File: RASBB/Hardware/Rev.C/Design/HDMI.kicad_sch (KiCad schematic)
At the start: 5 parts, among them IC11 TPD12S016PWR, J3 HDMI-001A

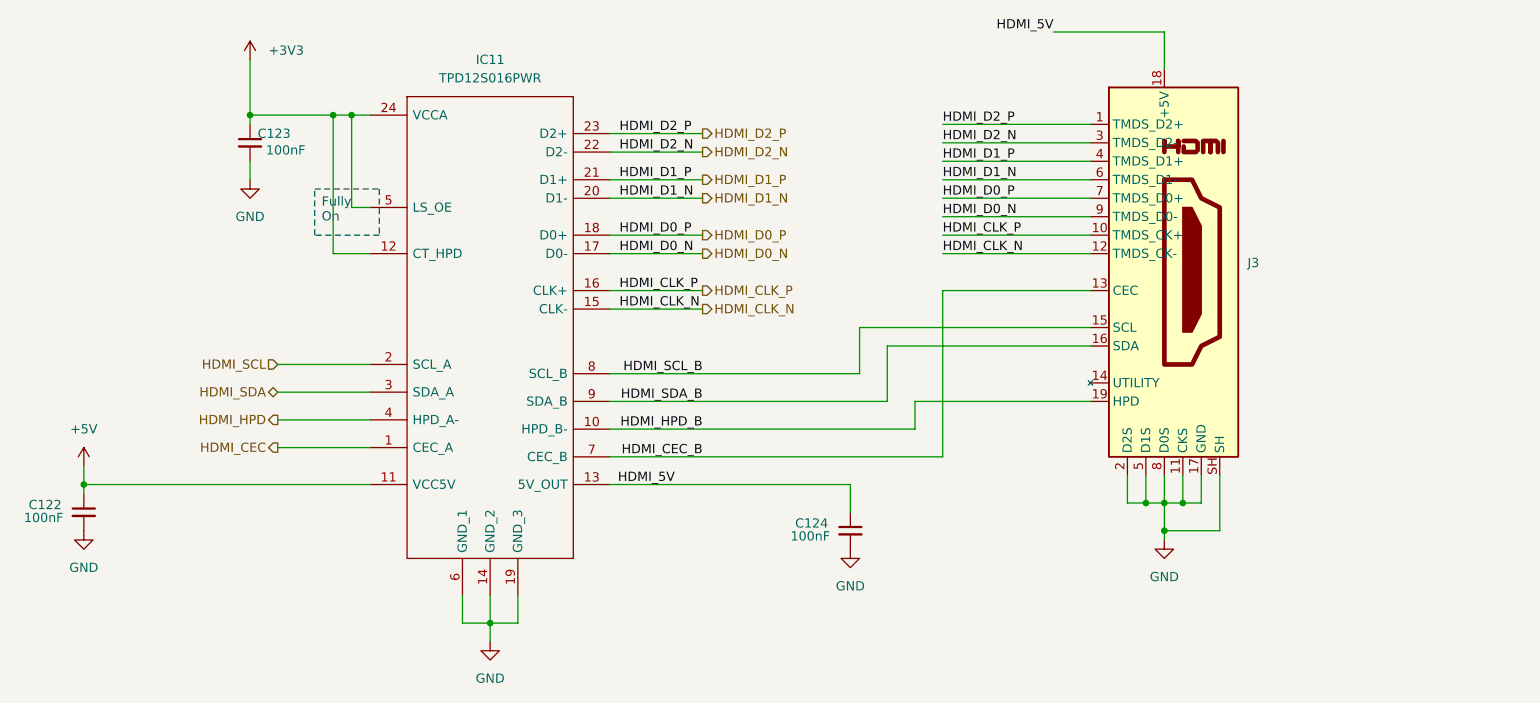
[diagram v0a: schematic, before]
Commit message: Draft AC
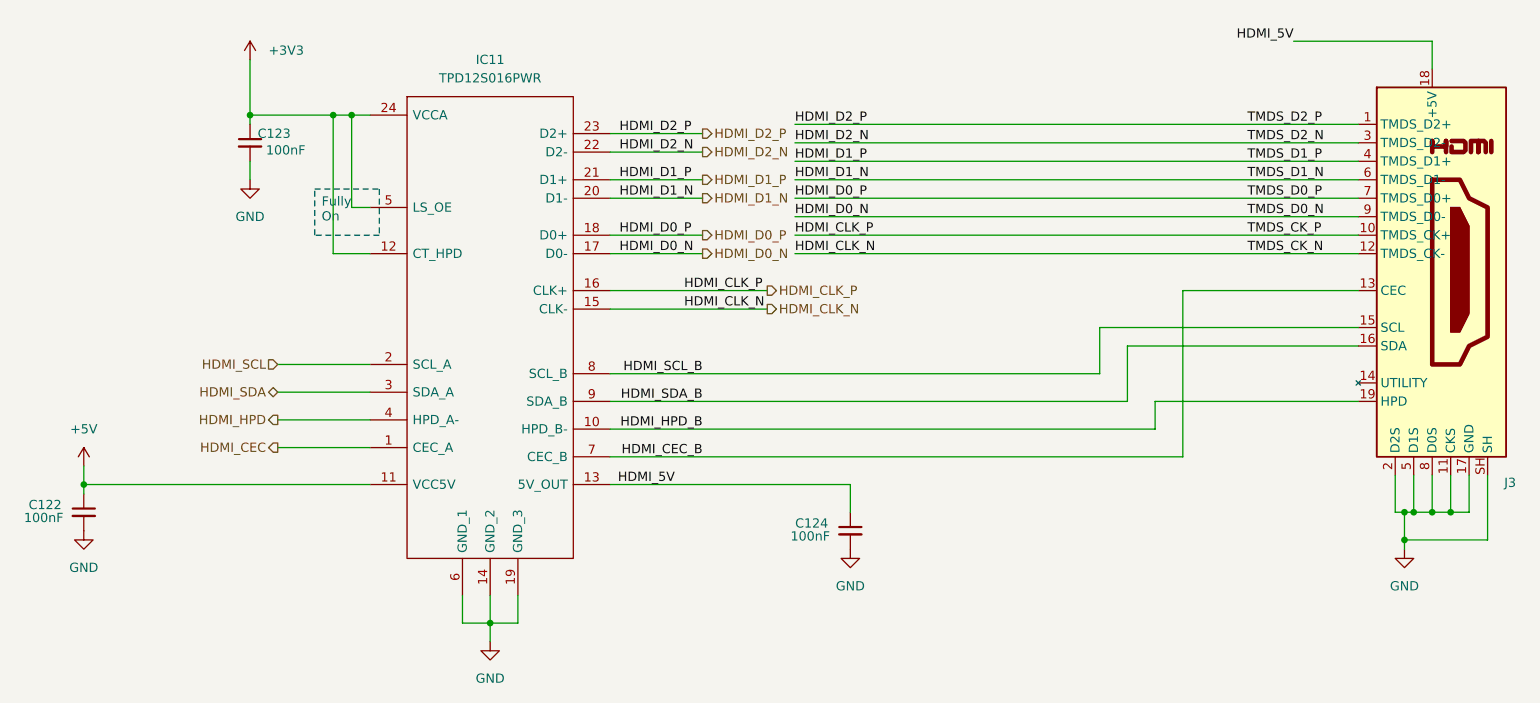
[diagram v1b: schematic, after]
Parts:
- IC11: LCSC Part #  C201665 -> (none)
- J3: LCSC Part #  C41347845 -> (none)
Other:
- moved on the sheet: J3
